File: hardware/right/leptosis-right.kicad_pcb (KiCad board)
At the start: 4 copper layers, 93.5 x 72.3 mm, 91 parts, among them J1 USB_C_Receptacle_USB2.0_14P, J2 Conn_01x02, Q2 2N7002, SW10 SW_Push, SW11 SW_Push, SW12 SW_Push, SW14 SW_Push, SW15 SW_Push, SW16 SW_Push, SW17 SW_Push, SW18 SW_Push, SW2 SW_Push, SW22 SW_Push, SW23 SW_Push, SW24 SW_Push, SW3 SW_Push, SW31 SW_SPDT, SW4 SW_Push, SW5 SW_Push, SW6 SW_Push, SW8 SW_Push, SW9 SW_Push, U1 nRF52840, U2 BQ24075RGT, U3 MAX17048X, Y1 32MHz 12pF, Y2 32.768kHz 12.5pF

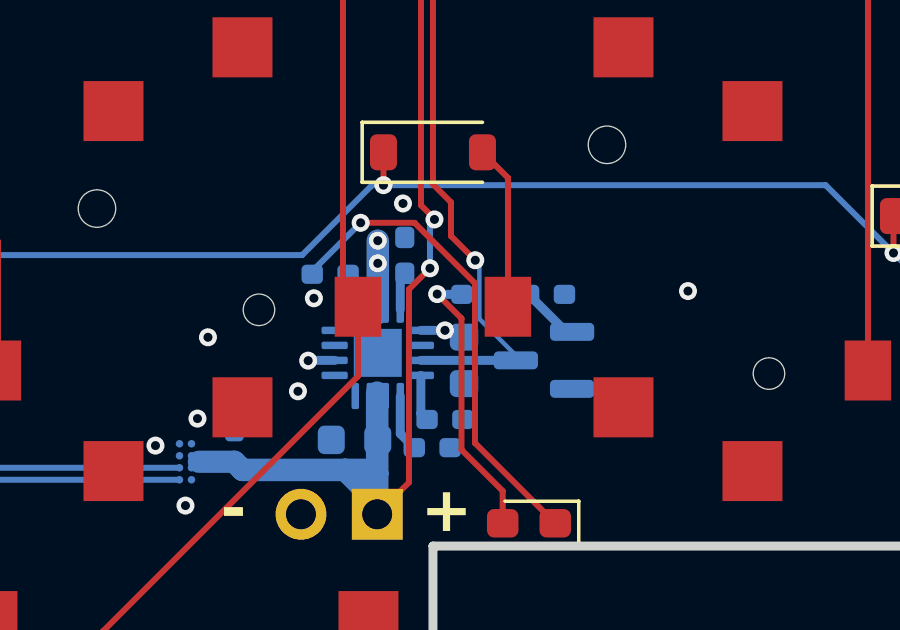
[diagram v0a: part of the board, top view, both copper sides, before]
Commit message: Finish
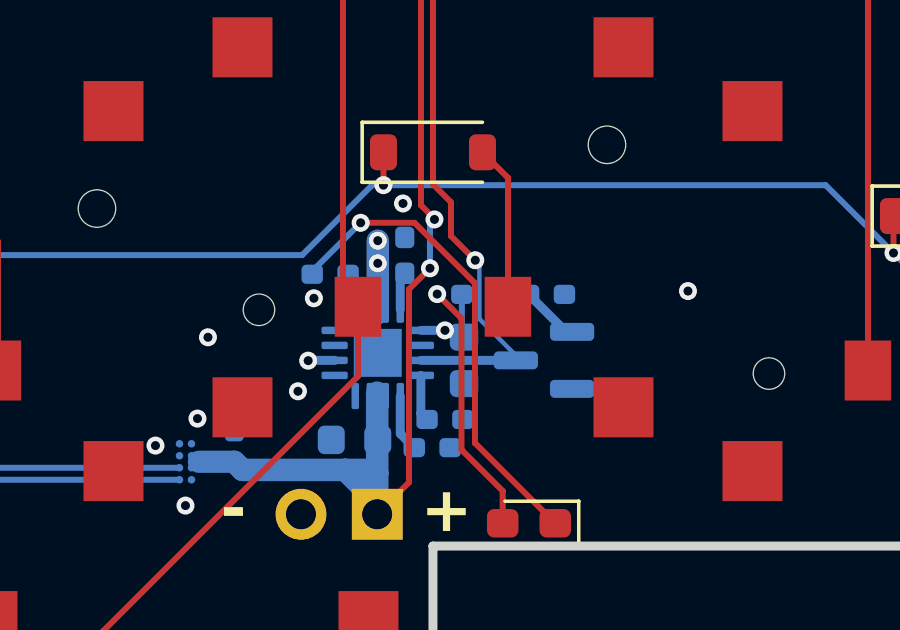
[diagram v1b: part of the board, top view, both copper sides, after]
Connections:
- R7 pad 2: +5V -> VBUS
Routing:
- net VBUS: track 11.1 -> 12.5 mm
- net +5V: track 16.0 -> 15.2 mm
